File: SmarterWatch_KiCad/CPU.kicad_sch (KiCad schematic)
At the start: 16 parts, among them SW1 SW_SPST, SW2 SW_SPST, U5 ESP32-C6-MINI-1

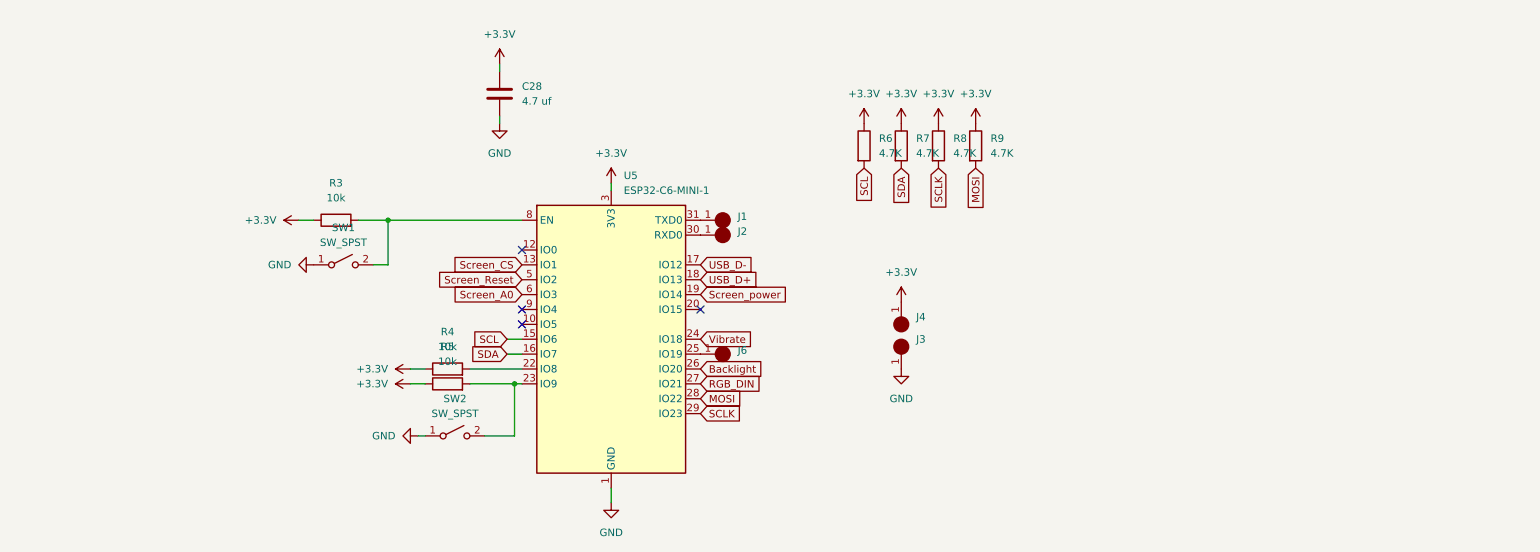
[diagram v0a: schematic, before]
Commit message: update
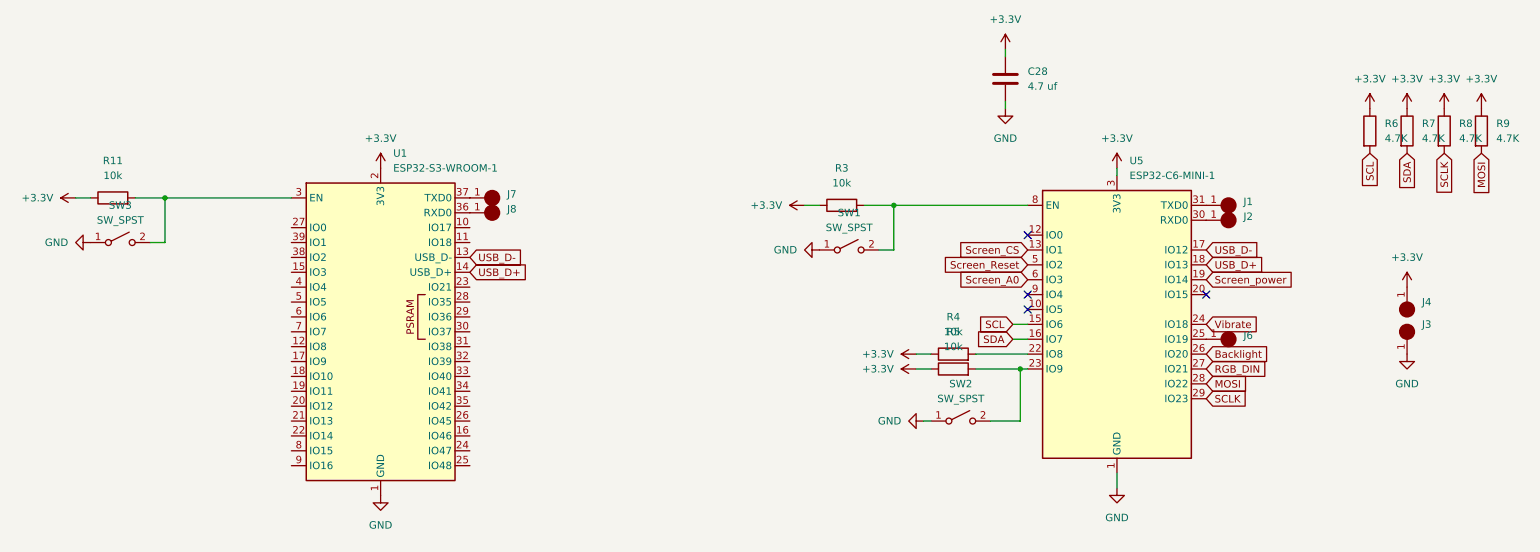
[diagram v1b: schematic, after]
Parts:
- added J7, J8: (no value), Connector_Wire:SolderWirePad_1x01_SMD_2x4mm, symbol SmarterWatch_symbols_j:Solder_pad
- added R11: 10k, Resistor_SMD:R_0402_1005Metric, symbol Device:R
- added SW3: SW_SPST, Custom_Foot:SMD_Button_6mm_SPST, symbol Switch:SW_SPST
- added U1: ESP32-S3-WROOM-1, RF_Module:ESP32-S3-WROOM-1, symbol RF_Module:ESP32-S3-WROOM-1
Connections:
- net +3.3V: now also R11.1, U1.2 (3V3)
- net GND: now also SW3.1 (A), U1.1 (GND), U1.40 (GND), U1.41 (GND)
- net USB_D+: now also U1.14 (USB_D+)
- net USB_D-: now also U1.13 (USB_D-)
- new net: J8.1, U1.36 (RXD0)
- new net: R11.2, SW3.2 (B), U1.3 (EN)
- new net: J7.1, U1.37 (TXD0)
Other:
- moved on the sheet: C28, J1, J2, J3, J4, J6, R3, R4, R5, R6, R7, R8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
